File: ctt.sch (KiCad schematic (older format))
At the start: 7 parts, among them CN1 CONN_3, CN2 CONN_3, J1 INDUCTOR

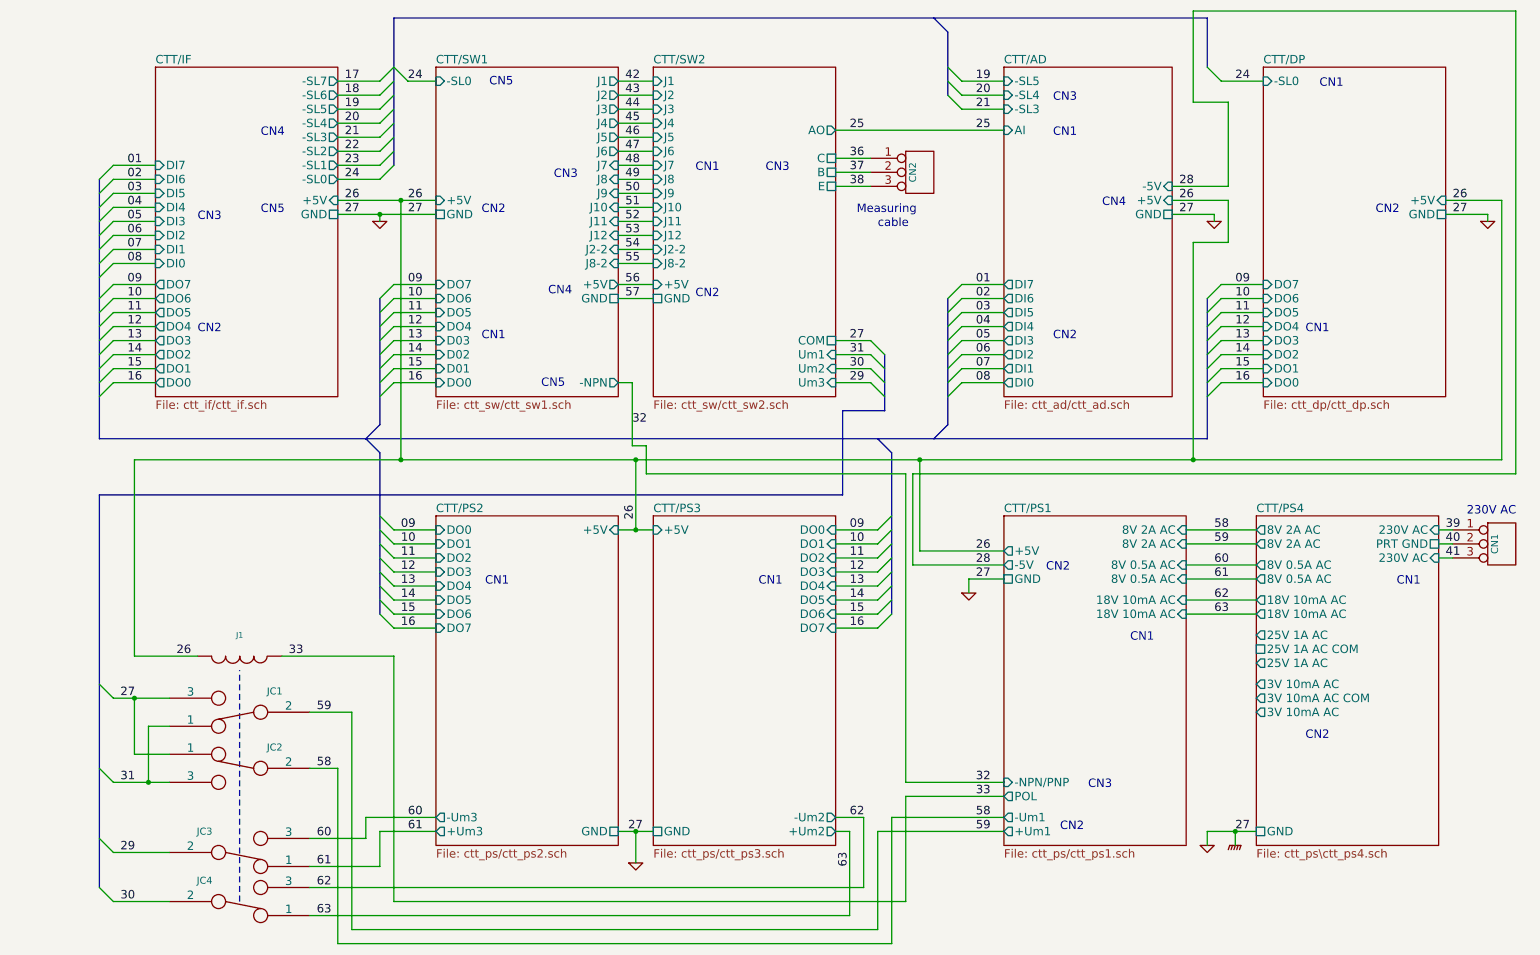
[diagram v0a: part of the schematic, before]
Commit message: 2011.05.26.esti állapot.
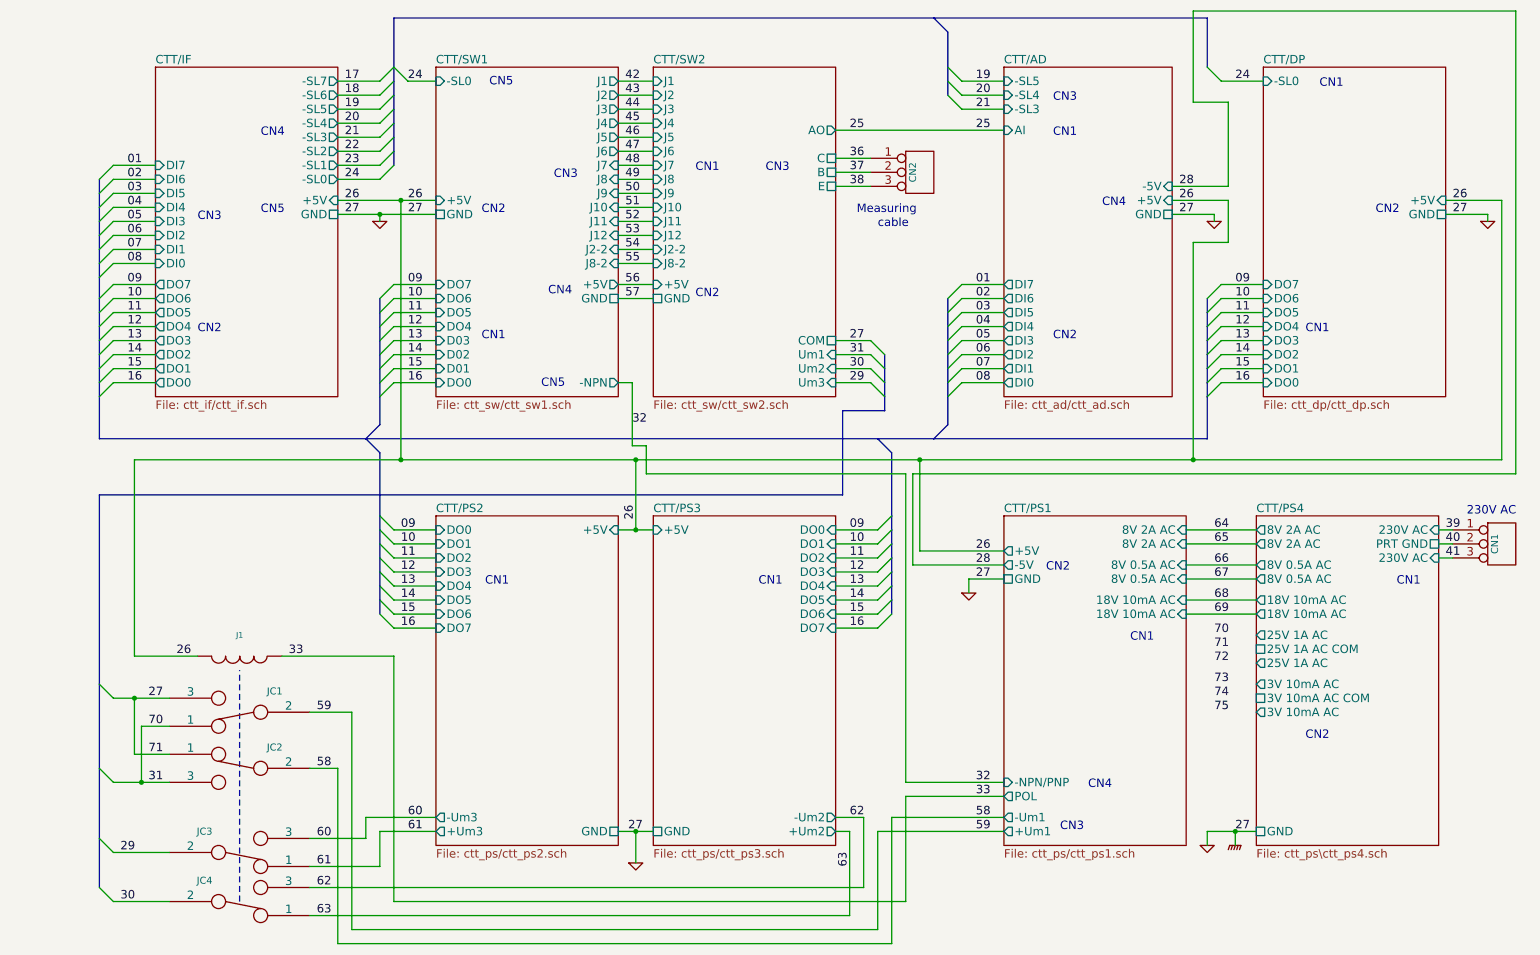
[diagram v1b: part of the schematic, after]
